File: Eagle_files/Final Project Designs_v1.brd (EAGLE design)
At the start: 100 x 80 mm, 29 parts, among them CON1 header, CON2 4PIN_GROVE_CONNECTORUNIVERSAL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, U1 TPS63000DRCR, U2 ATXMEGA32AA, X1 USB-MICROB", X4 JTAG, X5 BANANA_PLUG, X6 BANANA_PLUG

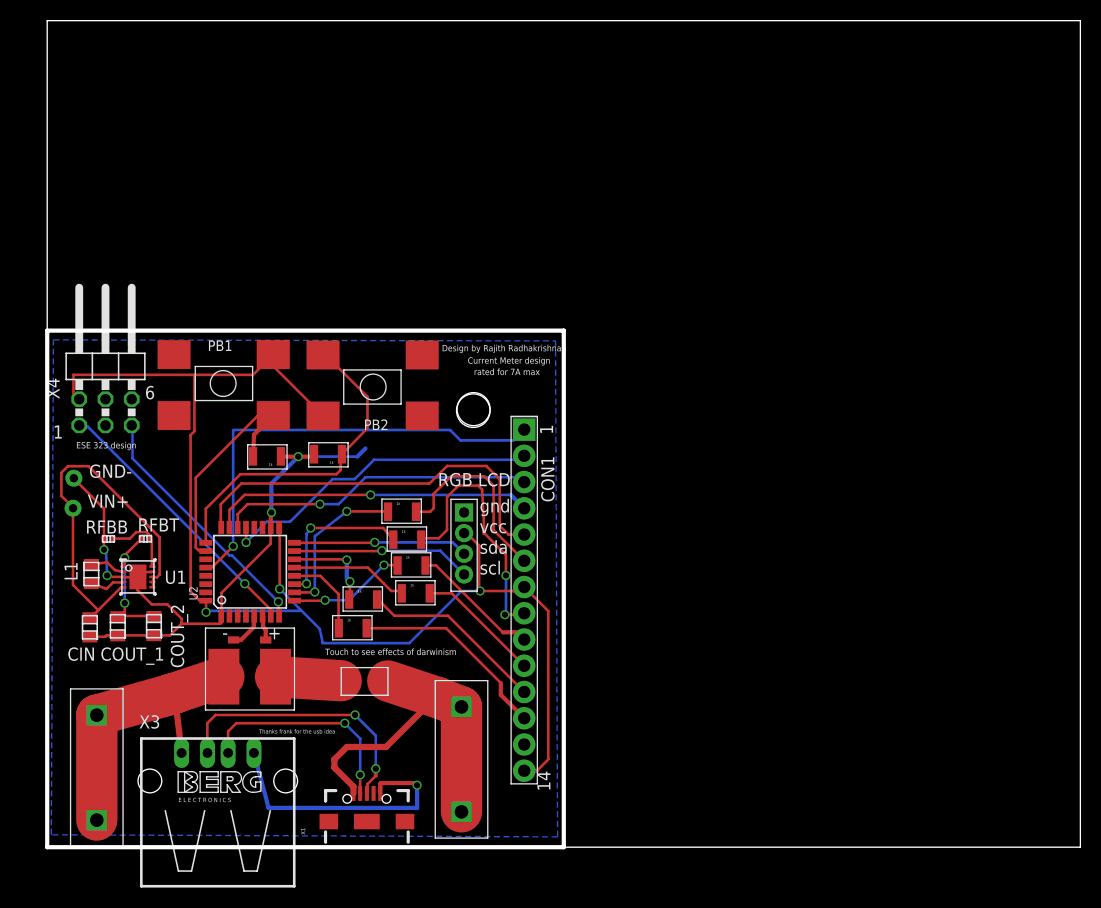
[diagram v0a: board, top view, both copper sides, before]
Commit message: finished everthing
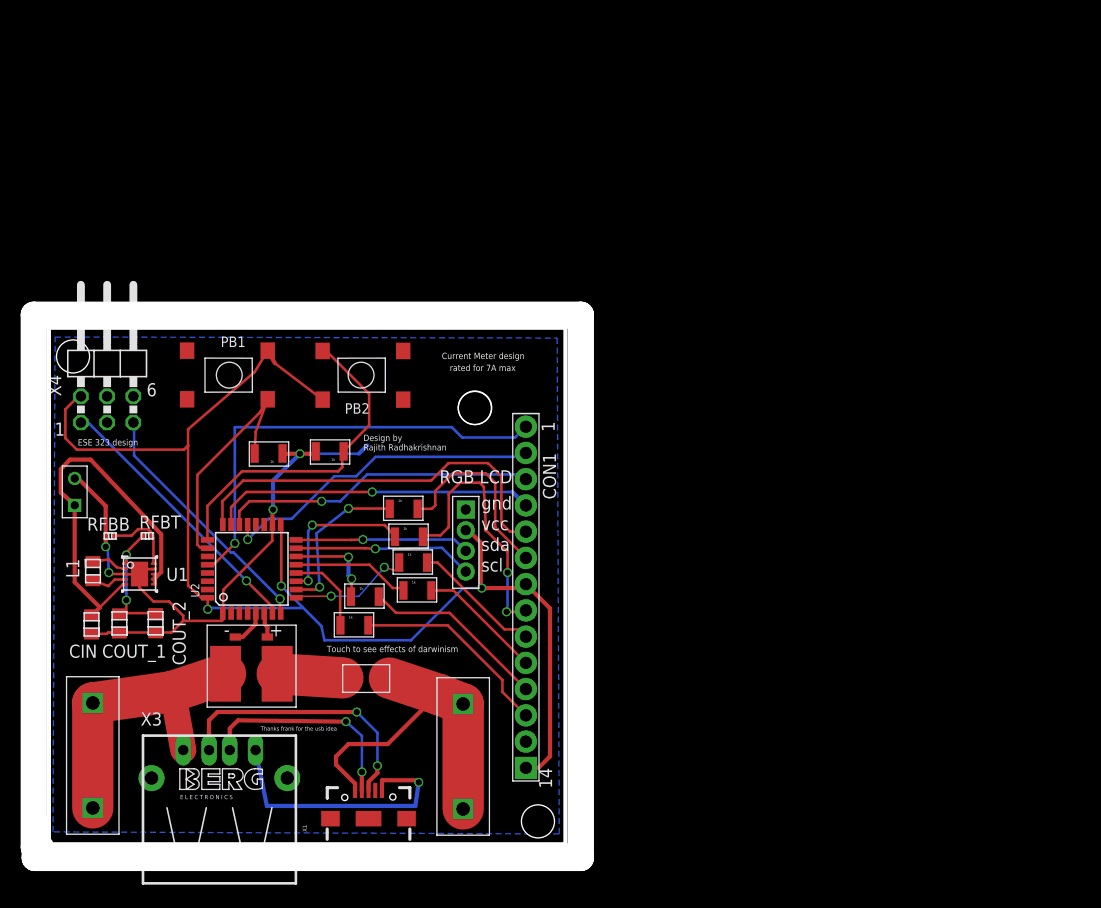
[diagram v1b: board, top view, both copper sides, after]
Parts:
- removed GND-, VIN+: TP-1502, sps:TP-1502
- added U$1: BATTERY, Tft_lcd_header:BATTERY
- moved PB2 2.43 mm to (29.2, 45.5)
- moved PB1 1.32 mm to (18.8, 45.9)
- moved X5 1.24 mm to (4.41, 8.88)
- moved R4 0.32 mm to (37.4, 24.1)
- moved R6 0.32 mm to (36.6, 29.2)
- moved COUT_1 0.32 mm to (6.99, 21.7)
- moved COUT_2 0.32 mm to (10.5, 21.7)
- moved F1 0.32 mm to (31.6, 15.5)
- moved R1 0.32 mm to (20.2, 19.5)
- moved R2 0.32 mm to (31.3, 20.7)
- moved R9 0.32 mm to (25.8, 39.1)
- moved RFBB 0.32 mm to (6.09, 30.1)
- moved RFBT 0.32 mm to (9.68, 30.1)
- moved U1 0.32 mm to (8.94, 26.4)
- moved U2 0.32 mm to (19.8, 26.9)
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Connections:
- net GND: now also U$1.GND; no longer GND-.1
- net VIN: now also U$1.VCC; no longer VIN+.1
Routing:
- net +3V3: track 126.4 -> 125.3 mm
- net VIN: track 37.4 -> 38.4 mm
- net B$2: track 29.3 -> 30.3 mm
- net N$10: track 22.6 -> 23.3 mm
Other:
- board size 100 x 80 mm -> 52.9 x 52.6 mm
- board text added: "https://radrajith.github.io/ESE_323_PCB_Design/"
- board text removed: "Thanks frank yee for usb idea, and taking the responsibility for ordering parts, pcb and taking in charge."
